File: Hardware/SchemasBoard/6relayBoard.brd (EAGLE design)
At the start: 53.1 x 41.8 mm, 47 parts, among them IC1 LNK304, IC3 MC33269ST-3.3T3, K1 FRS1B, K2 FRS1B, K3 FRS1B, K4 FRS1B, K5 FRS1B, K6 FRS1B, T1 BC846, T2 BC846, T3 BC846, T4 BC846, T5 BC846, T6 BC846

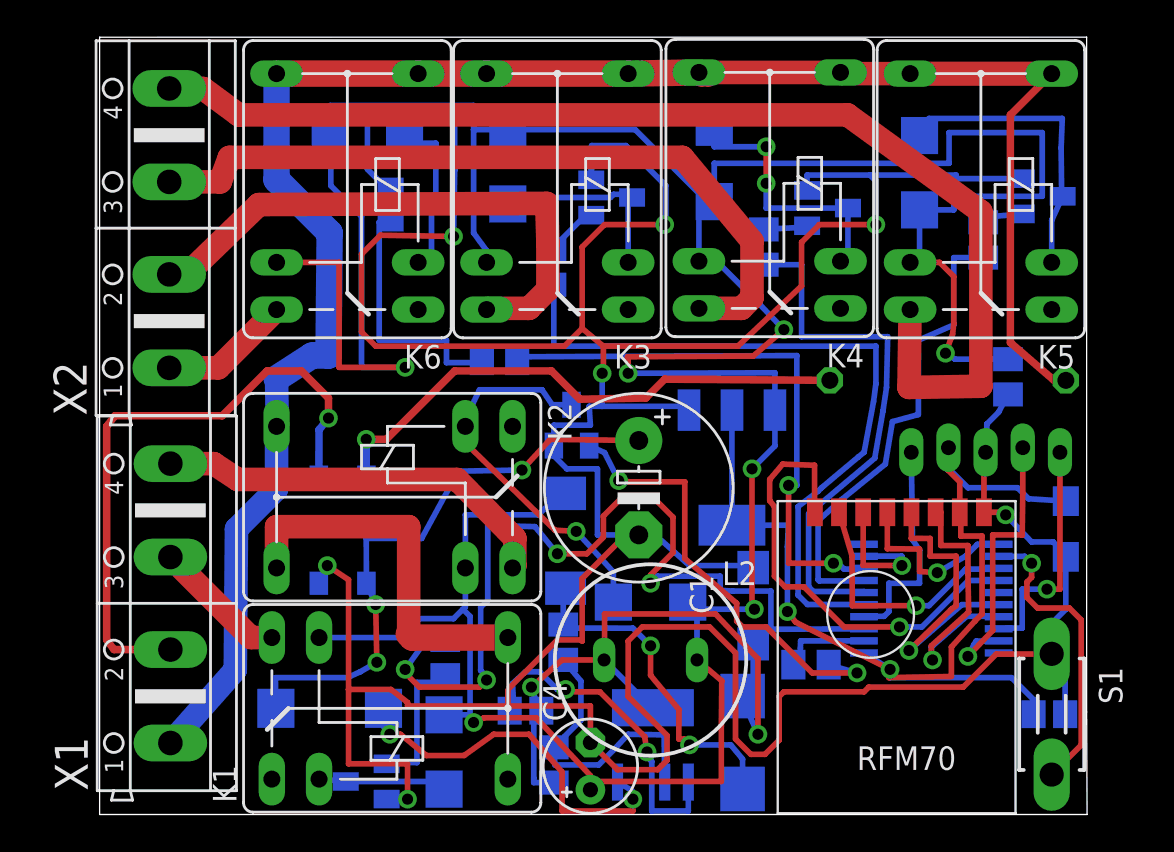
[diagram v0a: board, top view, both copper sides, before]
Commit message: fghf
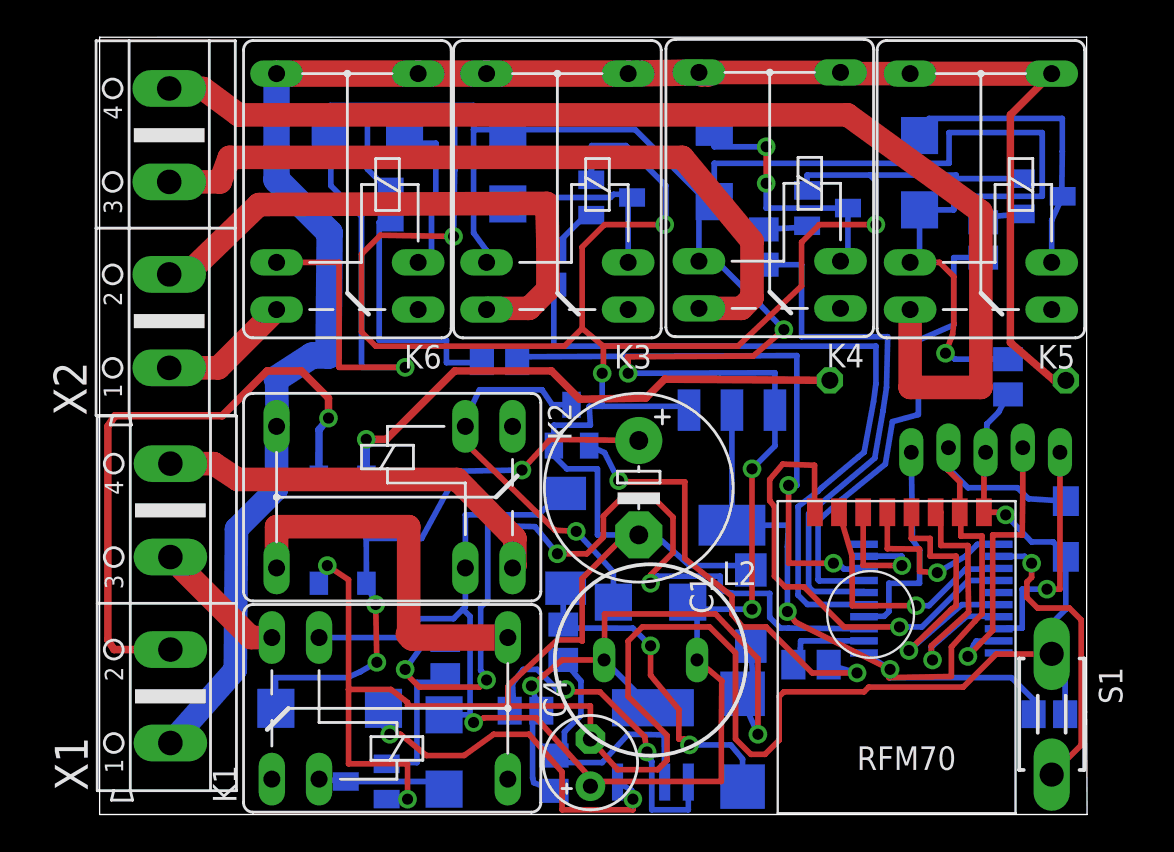
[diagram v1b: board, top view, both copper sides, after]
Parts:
- moved R4 0.44 mm to (23.3, 2.22)
- moved C4 0.19 mm to (25.3, 2.79)
- moved D3 0.18 mm to (33.9, 11.1)
- moved C3 0.13 mm to (33.5, 4.00)
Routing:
- net N$27: track 205.0 -> 204.4 mm
- net N$35: track 48.4 -> 47.9 mm

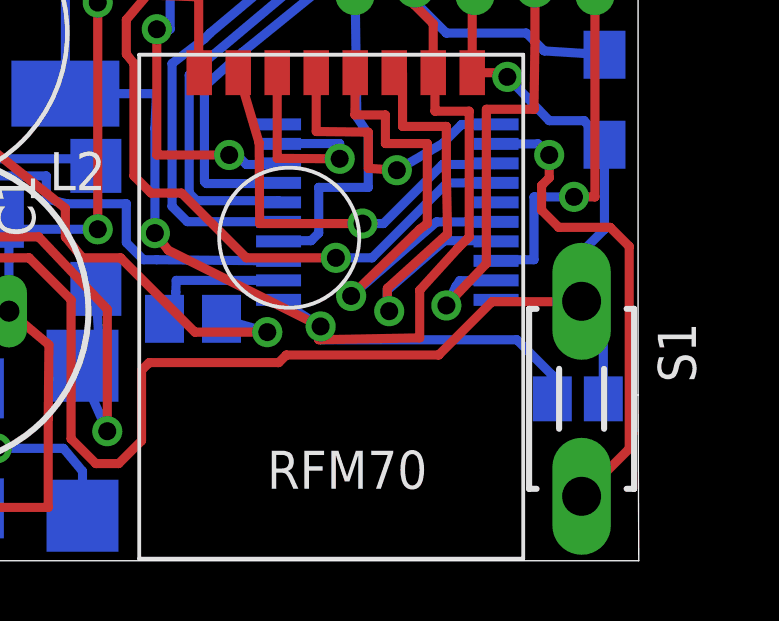
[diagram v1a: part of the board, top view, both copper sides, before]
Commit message: fixed bug.
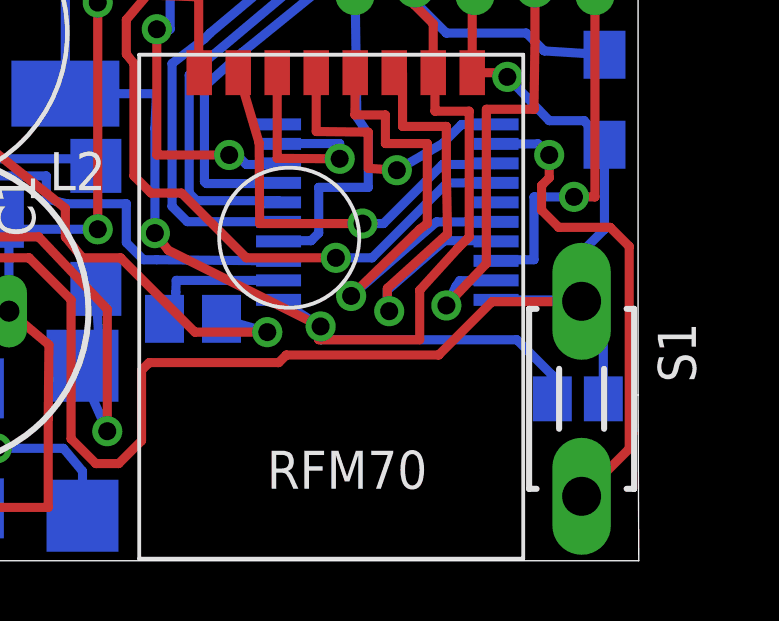
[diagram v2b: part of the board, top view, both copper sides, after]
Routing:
- net GND: track 236.0 -> 238.9 mm
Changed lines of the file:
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@@
 <?xml version="1.0" encoding="utf-8"?>
 <!DOCTYPE eagle SYSTEM "eagle.dtd">
-<eagle version="6.3">
+<eagle version="6.4">
 <drawing>
 <settings>
@@
 <wire x1="47.244" y1="21.6535" x2="46.609" y2="21.0185" width="0.3048" layer="16"/>
 <wire x1="46.609" y1="19.558" x2="46.5455" y2="19.4945" width="0.3048" layer="16"/>
-<wire x1="47.117" y1="8.636" x2="47.174" y2="8.6955" width="0" layer="19" extent="1-16"/>
+<wire x1="47.2495" y1="8.6955" x2="50.09" y2="8.6955" width="0.3048" layer="16"/>
+<wire x1="50.09" y1="8.6955" x2="50.09" y2="8.636" width="0.3048" layer="16"/>
 </signal>
 <signal name="N$11">
@@
 <wire x1="41.402" y1="7.8105" x2="40.5115" y2="8.382" width="0.3048" layer="16"/>
 <wire x1="40.5115" y1="8.382" x2="39.9995" y2="8.6955" width="0.3048" layer="16"/>
-<wire x1="44.704" y1="7.4295" x2="41.3385" y2="7.366" width="0.3048" layer="1"/>
+<wire x1="44.704" y1="7.366" x2="41.3385" y2="7.366" width="0.3048" layer="1"/>
 <wire x1="41.3385" y1="7.366" x2="41.3385" y2="7.6835" width="0.3048" layer="1"/>
 <wire x1="41.3385" y1="7.6835" x2="41.402" y2="7.8105" width="0.3048" layer="1"/>
 <wire x1="45.974" y1="10.414" x2="44.704" y2="9.017" width="0.3048" layer="1"/>
-<wire x1="44.704" y1="9.017" x2="44.704" y2="7.4295" width="0.3048" layer="1"/>
+<wire x1="44.704" y1="9.017" x2="44.704" y2="7.366" width="0.3048" layer="1"/>
 <wire x1="45.155" y1="16.2685" x2="45.155" y2="17.9005" width="0.3048" layer="1"/>
 <wire x1="45.155" y1="17.9005" x2="44.5135" y2="18.542" width="0.3048" layer="1"/>
